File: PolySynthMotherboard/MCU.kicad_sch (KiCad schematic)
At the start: 13 parts, among them U201 STM32F411RETx, U202 74HC595, U203 74HC595

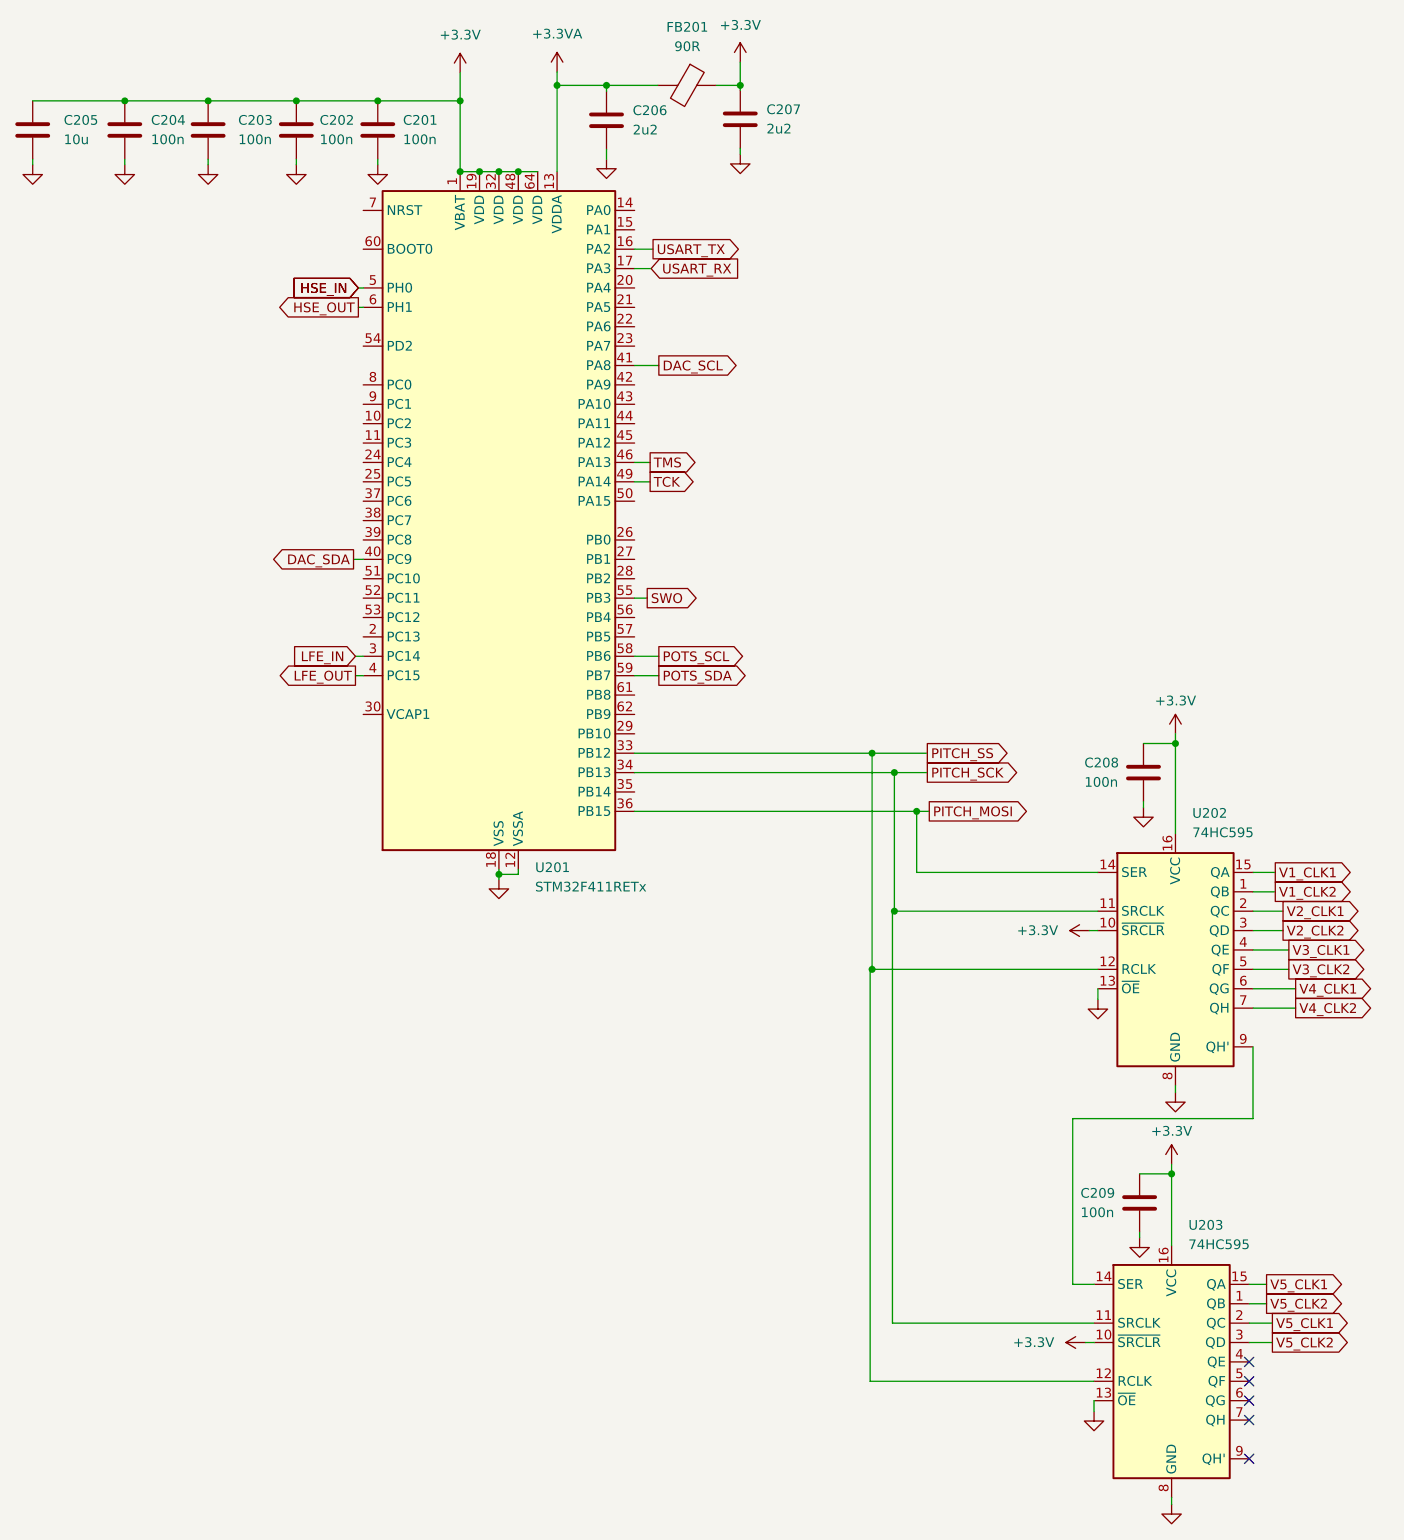
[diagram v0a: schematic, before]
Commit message: motherboard hardware
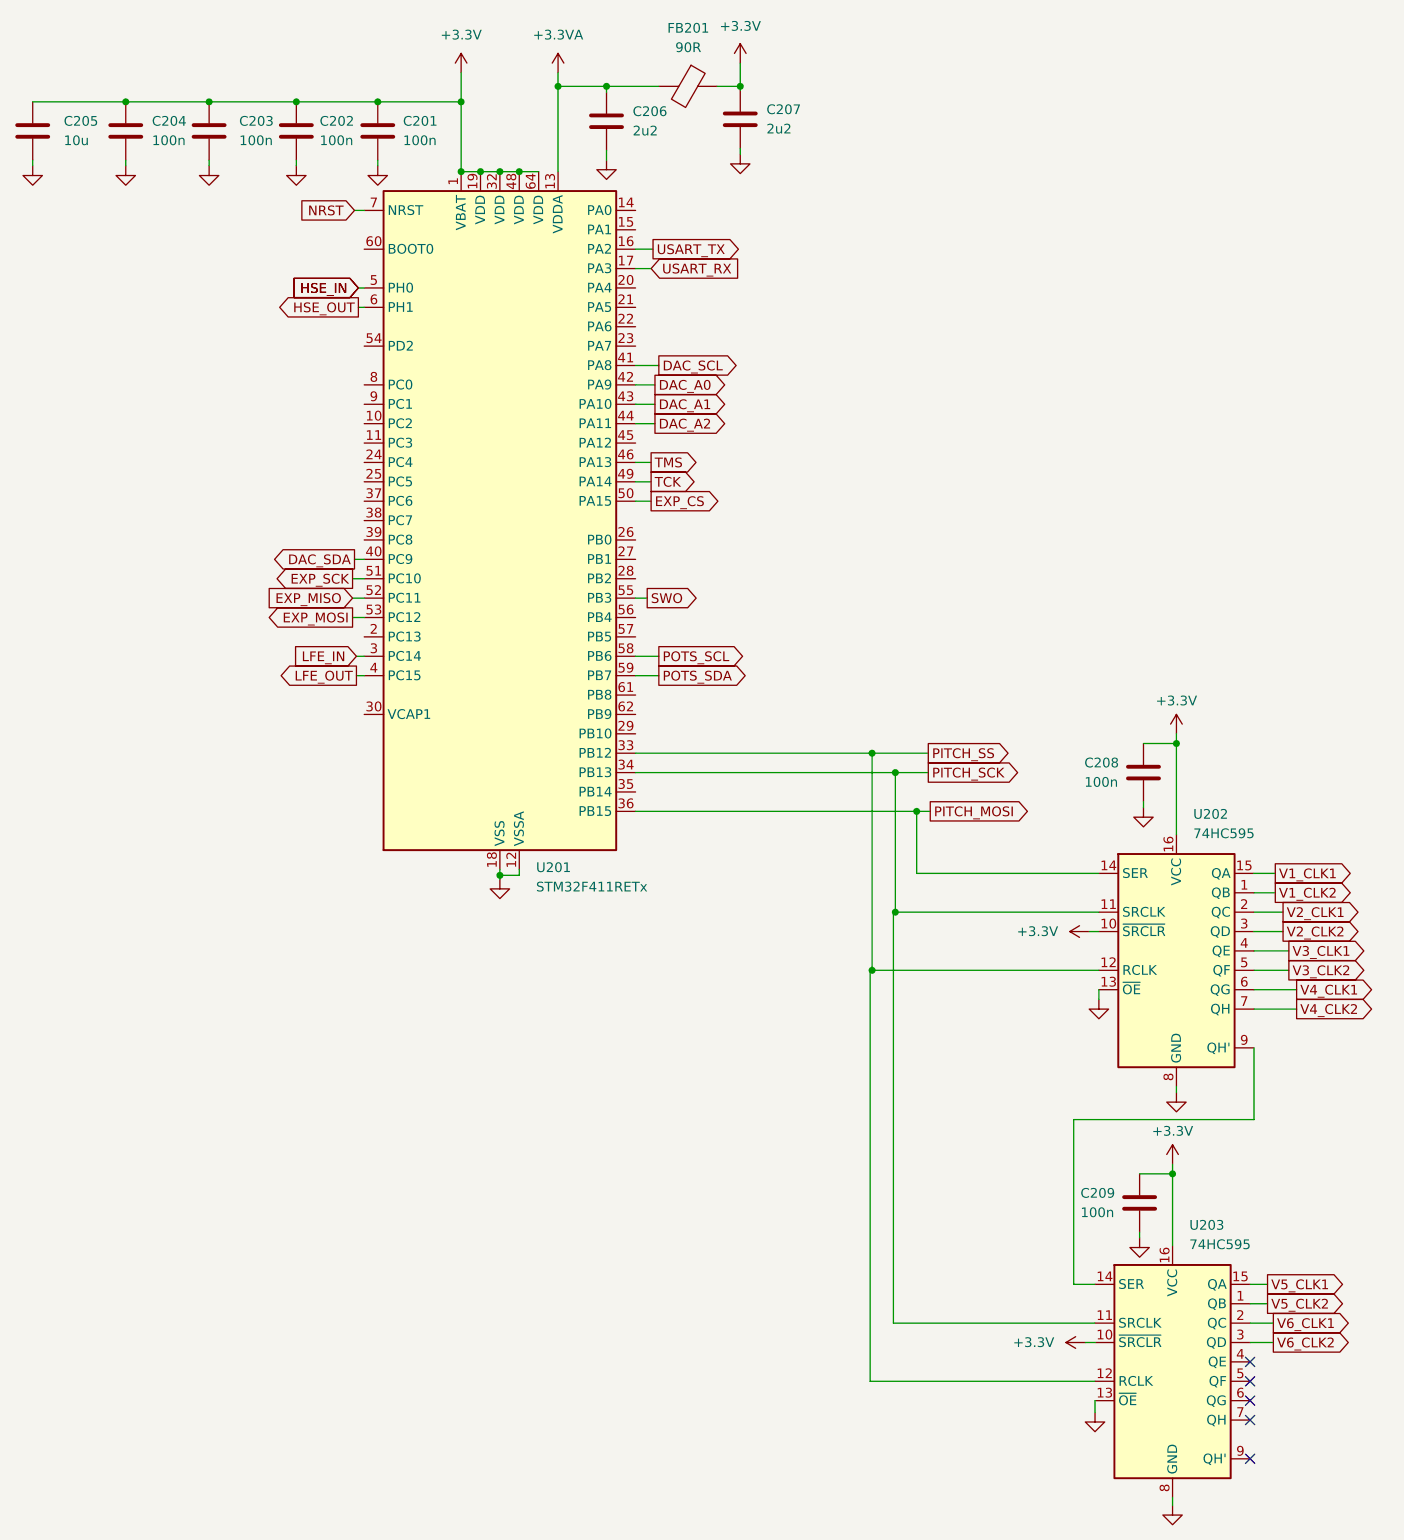
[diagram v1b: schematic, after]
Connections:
- net V5_CLK1: no longer U203.2 (QC)
- net V5_CLK2: no longer U203.3 (QD)
- net DAC_A0: now reaches U201.42 (PA9)
- net DAC_A1: now reaches U201.43 (PA10)
- net DAC_A2: now reaches U201.44 (PA11)
- net EXP_CS: now reaches U201.50 (PA15)
- net EXP_SCK: now reaches U201.51 (PC10)
- net EXP_MISO: now reaches U201.52 (PC11)
- net EXP_MOSI: now reaches U201.53 (PC12)
- net NRST: now reaches U201.7 (NRST)
- new net V6_CLK1: U203.2 (QC)
- new net V6_CLK2: U203.3 (QD)
